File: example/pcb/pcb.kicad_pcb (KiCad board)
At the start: 2 copper layers, 10 parts, among them IC1 AD8403ARUZ1-REEL, IC2 AD8403ARUZ1-REEL, J1 Conn_01x06_Pin, J2 Conn_01x06_Pin, J3 Conn_01x05_Pin

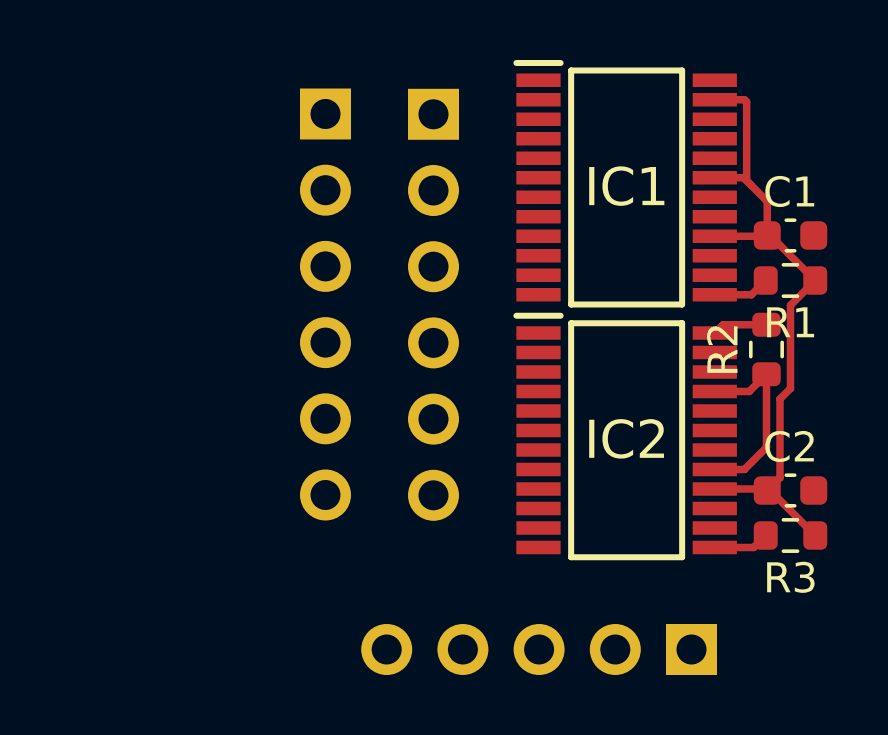
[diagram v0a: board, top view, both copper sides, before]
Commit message: Update pcb
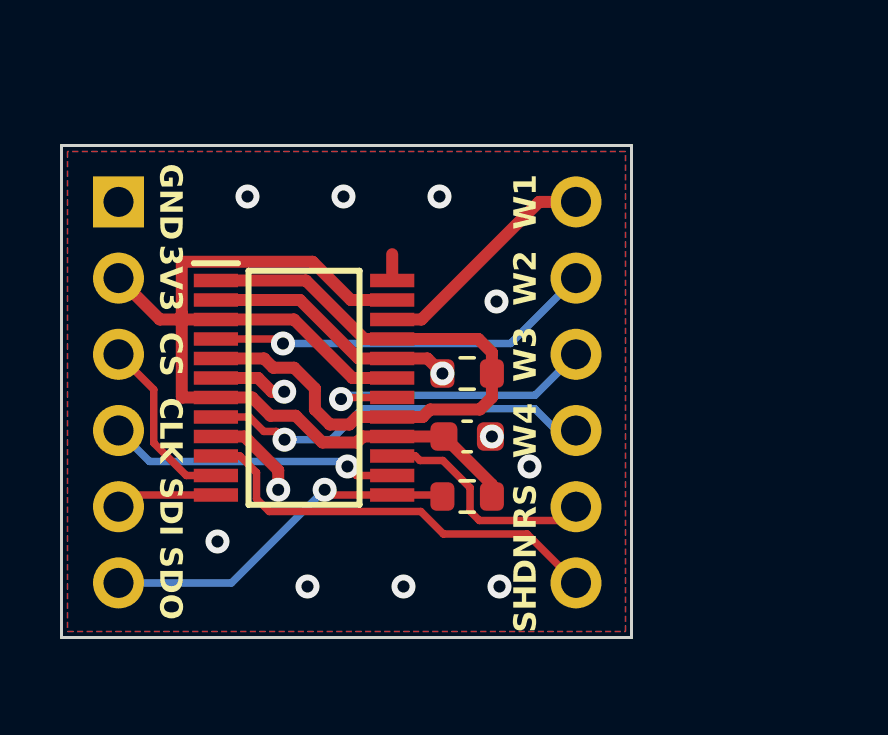
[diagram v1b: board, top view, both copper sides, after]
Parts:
- removed C2: 100n, Capacitor_SMD:C_0603_1608Metric
- removed IC2: AD8403ARUZ1-REEL, AD8403ARUZ1-REEL:SOP65P640X120-24N
- removed J3: Conn_01x05_Pin, Connector_PinHeader_2.54mm:PinHeader_1x05_P2.54mm_Vertical
- removed R3: 10k, Resistor_SMD:R_0603_1608Metric
- moved R1 13.0 mm to (78.3, 43.8)
- moved C1 12.7 mm to (78.3, 41.8)
- moved IC1 12.7 mm to (72.9, 40.2)
- moved J2 10.9 mm to (66.7, 34.0)
- moved R2 10.0 mm to (78.3, 39.7), turned to 180 degrees
- moved J1 8.85 mm to (82.0, 34.0)
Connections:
- net W1_1 renamed W1
- net W2_1 renamed W2
- net W3_1 renamed W3
- net W4_1 renamed W4
- IC1 pad 10: SHDN_1 -> SHDN
- IC1 pad 13: Net-(IC1-SDO) -> SDO
- IC1 pad 15: RS_1 -> RS
- J1 pad 5: SHDN_1 -> RS
- J1 pad 6: RS_1 -> SHDN
- J2 pad 1: W1_2 -> B_GND
- J2 pad 2: W2_2 -> A_3V3
- J2 pad 3: W3_2 -> CS
- J2 pad 4: W4_2 -> CLK
- J2 pad 5: SHDN_2 -> SDI
- J2 pad 6: RS_2 -> SDO
- R1 pad 2: Net-(IC1-SDO) -> SDO
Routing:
- net AGND: track 6.43 -> 22.6 mm
- net SHDN: track 0.00 -> 14.3 mm
- net B_GND: track 1.84 -> 15.2 mm, vias 0 -> 13
- net W4: track 0.00 -> 13.0 mm, vias 0 -> 1
- net W2: track 0.00 -> 13.0 mm, vias 0 -> 1
- net SDO: track 0.00 -> 12.2 mm, vias 0 -> 1
- net A_3V3: track 22.7 -> 34.9 mm
- net W3: track 0.00 -> 10.2 mm, vias 0 -> 1
- net CLK: track 0.00 -> 9.74 mm, vias 0 -> 1
- net W1: track 0.00 -> 7.75 mm
- net RS: track 0.00 -> 7.67 mm
- net CS: track 0.00 -> 5.96 mm
- net SDI: track 0.00 -> 3.41 mm
- net Net-(IC1-SDO): track 1.90 -> 0.00 mm
- net Net-(IC2-SDO): track 1.86 -> 0.00 mm
- added copper zone on B.Cu, net B_GND
- added copper zone on F.Cu, net B_GND
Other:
- board outline added: 19 x 16.4 mm
- board text added: "3V3"
- board text added: "CLK"
- board text added: "CS"
- board text added: "GND"
- board text added: "JLCJLCJLCJLC"
- board text added: "RS"
- board text added: "SDI"
- board text added: "SDO"
- board text added: "SHDN"
- board text added: "W1"
- board text added: "W2"
- board text added: "W3"
- board text added: "W4"
